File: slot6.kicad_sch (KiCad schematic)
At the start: 1 part

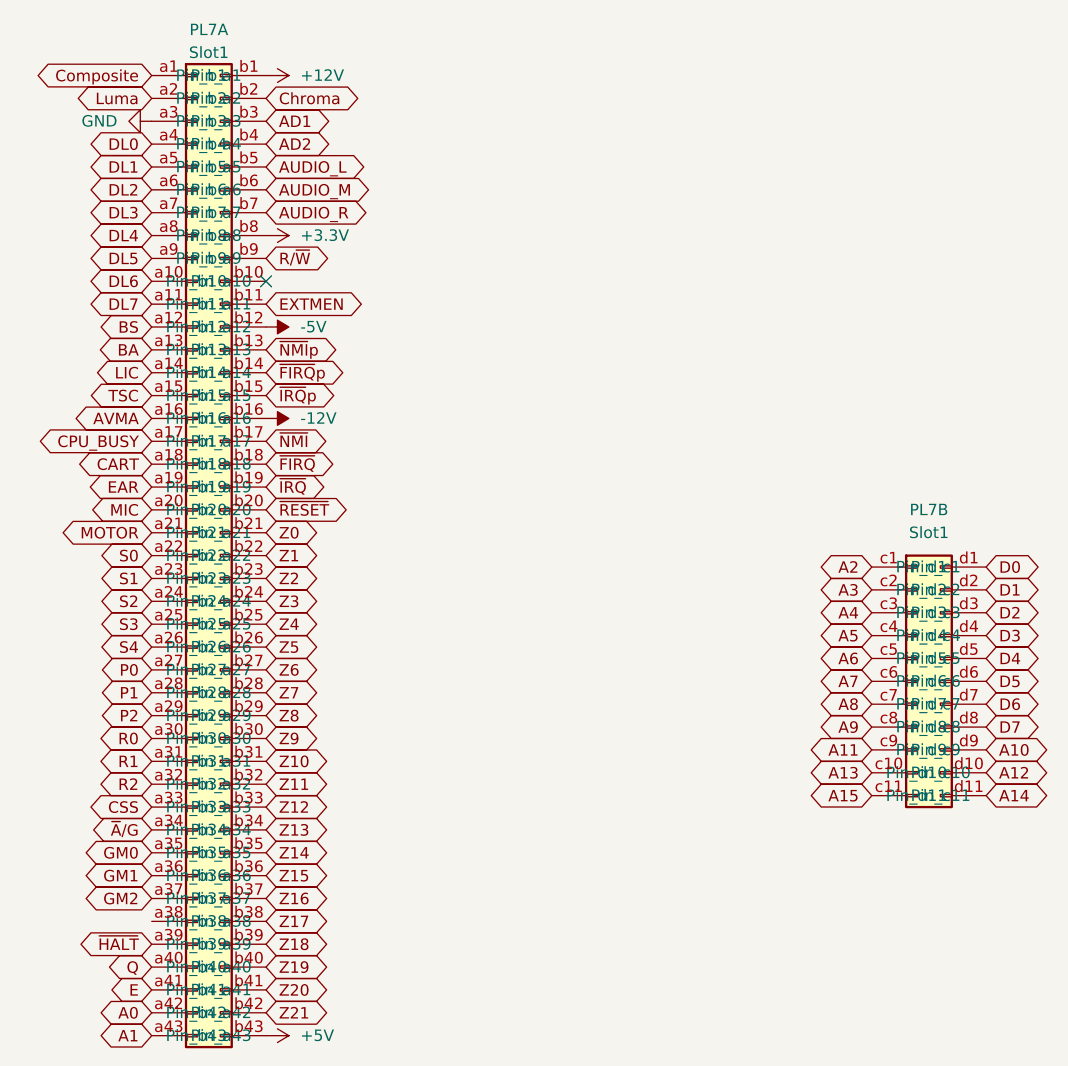
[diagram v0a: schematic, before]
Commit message: board layout
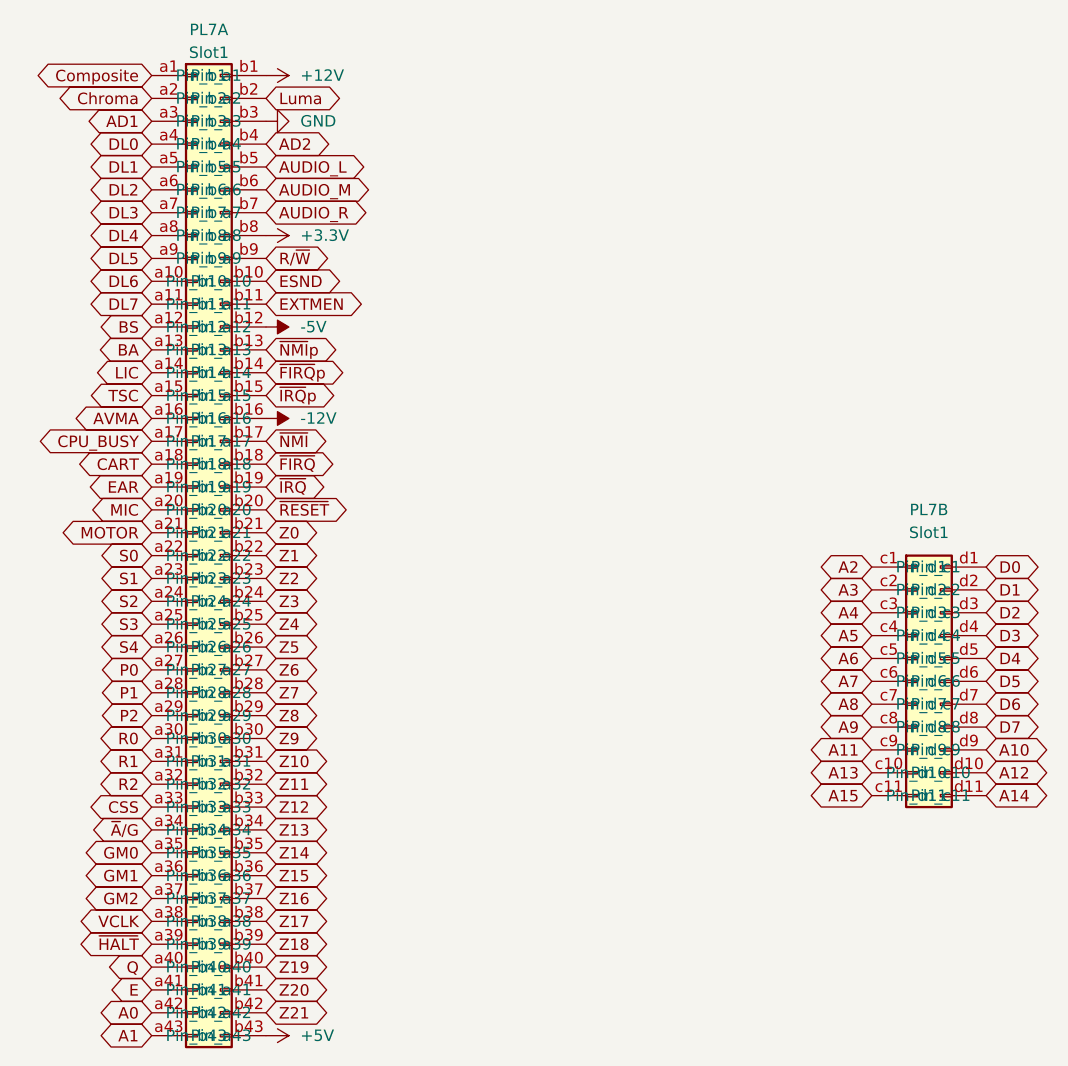
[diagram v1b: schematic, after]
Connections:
- net AD1: now also PL7.a3 (Pin_a3); no longer PL7.b3 (Pin_b3)
- net Chroma: now also PL7.a2 (Pin_a2); no longer PL7.b2 (Pin_b2)
- net GND: now also PL7.b3 (Pin_b3); no longer PL7.a3 (Pin_a3)
- net Luma: now also PL7.b2 (Pin_b2); no longer PL7.a2 (Pin_a2)
- net VCLK: now reaches PL7.a38 (Pin_a38)
- net ESND: now reaches PL7.b10 (Pin_b10)
- no-connect marks 1 -> 0
